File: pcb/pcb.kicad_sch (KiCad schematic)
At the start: 31 parts, among them J1 Screw_Terminal_01x02, K00 Kailh Choc, K01 Kailh Choc, K02 Kailh Choc, K10 Kailh Choc, K11 Kailh Choc, K12 Kailh Choc, K20 Kailh Choc, K21 Kailh Choc, K22 Kailh Choc, K23 Kailh Choc, K30 Kailh Choc, K31 Kailh Choc, K32 Kailh Choc, K33 Kailh Choc, K40 Kailh Choc, K41 Kailh Choc, K42 Kailh Choc, K43 Kailh Choc, K50 Kailh Choc, K51 Kailh Choc, K52 Kailh Choc, K53 Kailh Choc, K60 Kailh Choc, SW1 SW_DPST, SW2 SW_SPDT, U1 nice_nano

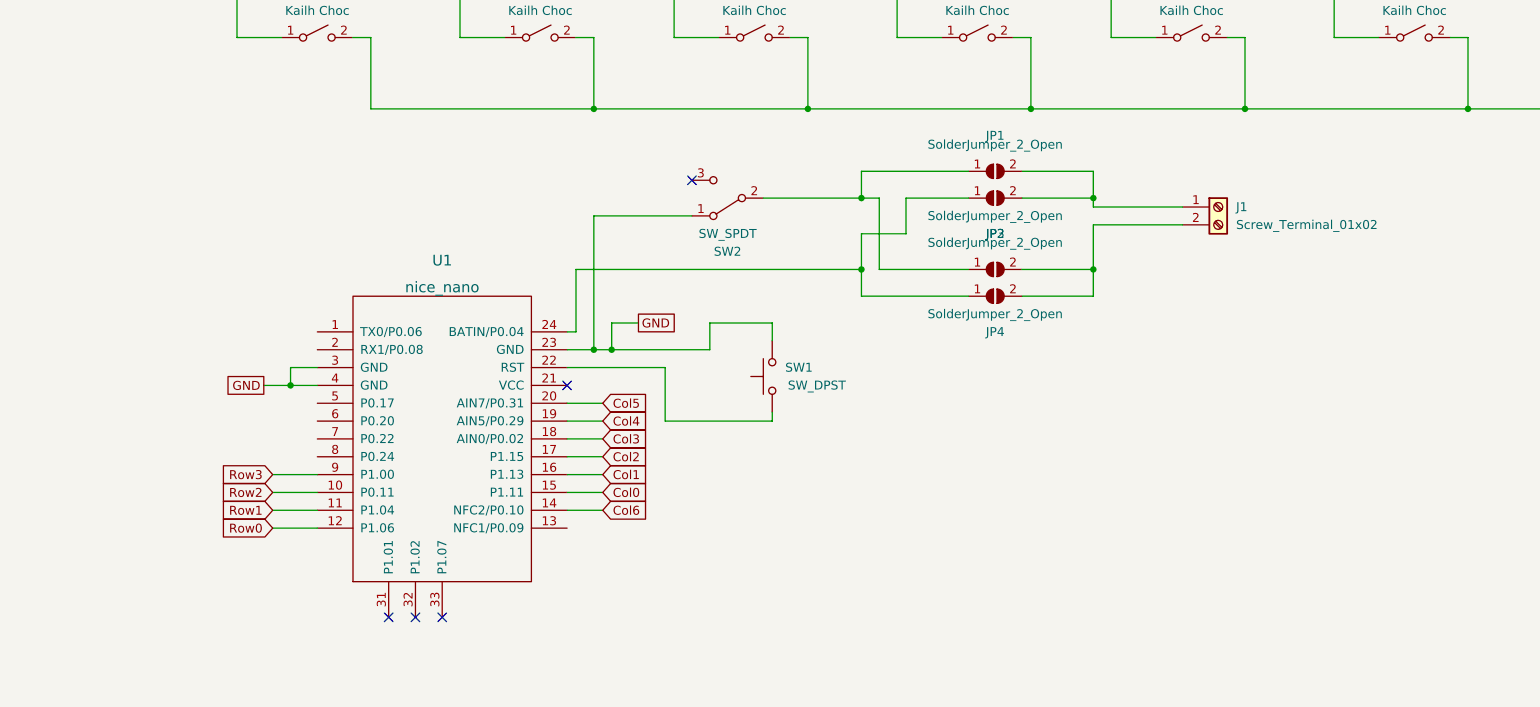
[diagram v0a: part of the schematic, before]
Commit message: update pcb
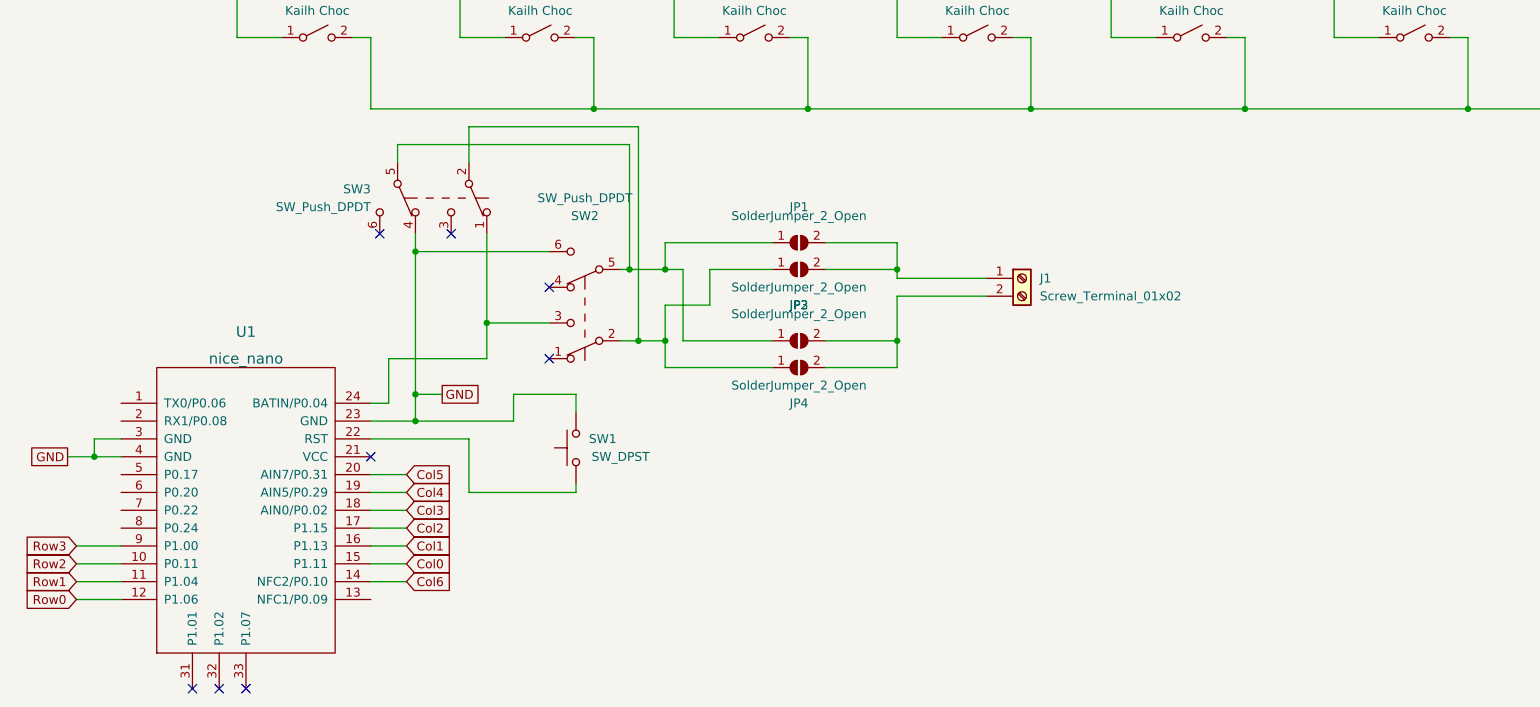
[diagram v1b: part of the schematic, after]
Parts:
- removed SW2: SW_SPDT, Button_Switch_SMD:SW_SPDT_CK-JS102011SAQN, symbol Switch:SW_SPDT
- added SW2, SW3: SW_Push_DPDT, lib:SW_JS202011SCQN (Reverse Mount), symbol Switch:SW_Push_DPDT
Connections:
- net GND: now also SW2.6 (C), SW3.4 (A)
- net at JP1.1 (A), JP3.1 (A): now also SW2.5 (B), SW3.5 (B)
- net at JP2.1 (A), JP4.1 (A): now also SW2.2 (B), SW3.2 (B); no longer U1.24 (BATIN/P0.04)
- new net: SW2.3 (C), SW3.1 (A), U1.24 (BATIN/P0.04)
- no-connect marks 5 -> 8
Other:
- moved on the sheet: J1, JP1, JP2, JP3, JP4, SW1, U1
